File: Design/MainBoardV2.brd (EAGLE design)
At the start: 76.8 x 71.1 mm, 110 parts, among them IC1 FT230XS, T1 NDS352AP, U1 STM32F20XR, U2 MicroSDCard

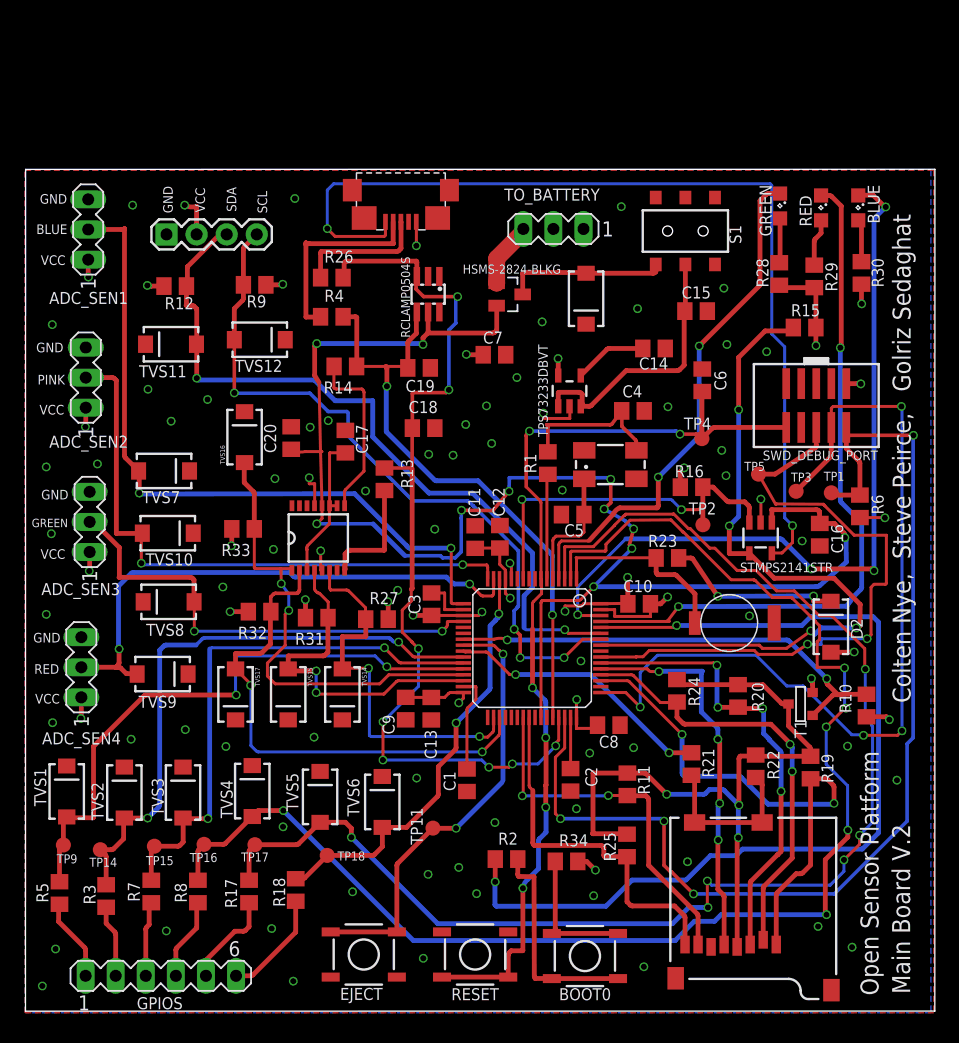
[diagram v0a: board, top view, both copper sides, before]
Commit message: Modified revision of board and schematic
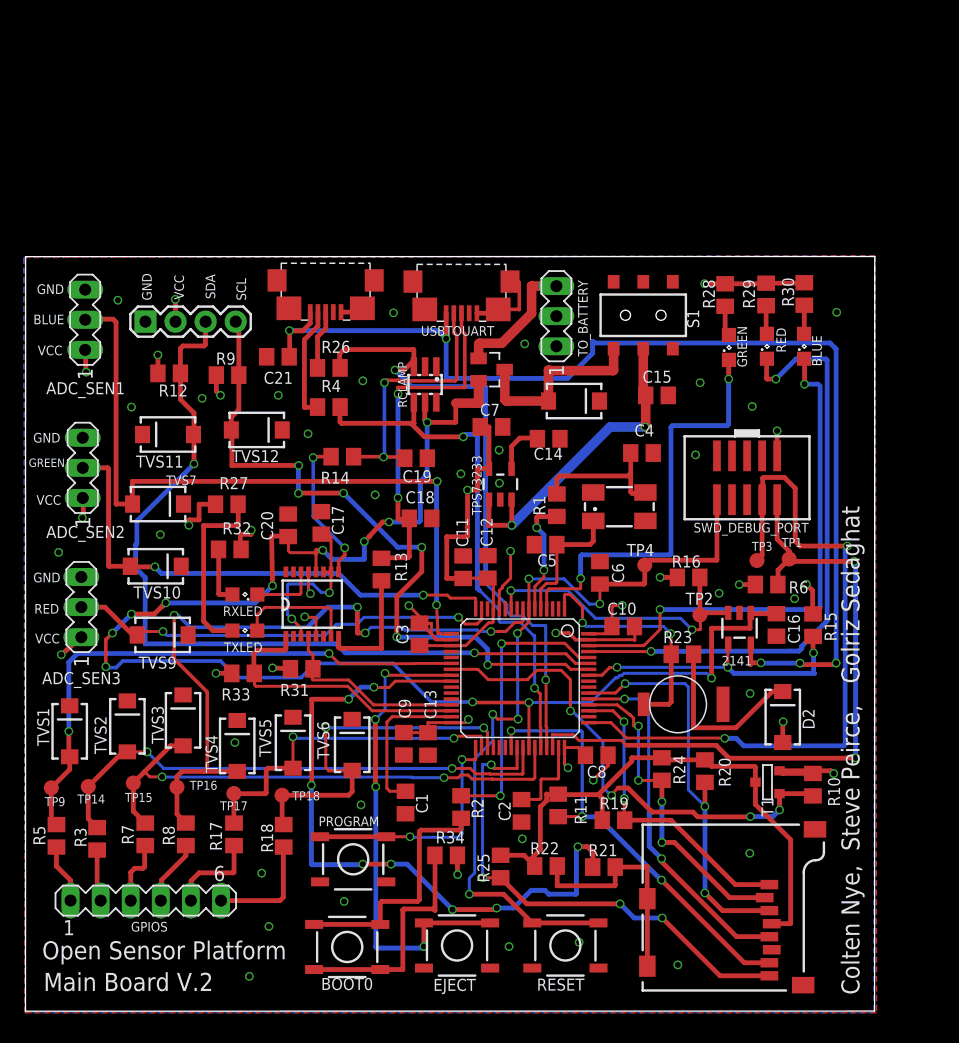
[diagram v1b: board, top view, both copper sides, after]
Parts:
- removed ADC_SEN4: (no value), con-lstb:MA03-1
- removed RCLAMP0504S: (no value), microbuilder:BREAKOUT_SOT23-6
- removed STMPS2141STR: (no value), microbuilder:SOT23-5
- removed TP11, TP5: TPB1,27, testpad:B1,27
- removed TPS73233DBVT: 3.3V, SparkFun-PowerIC:SOT23-5
- removed TVS14, TVS15, TVS16, TVS17, TVS8: TVS, SparkFun-DiscreteSemi:SMA-DIODE
- added 2141: (no value), microbuilder:SOT23-5
- added C21: 10u, rcl:C0805
- added PROGRAM: Program, SparkFun-Electromechanical:TACTILE-SWITCH-SMD
- added RCLAMP: (no value), microbuilder:BREAKOUT_SOT23-6
- added RXLED, TXLED: (no value), led:SML0805
- added TPS73233: 3.3V, SparkFun-PowerIC:SOT23-5
- added USBTOUART: USB_Shield, con-hirose:ZX62R-B-5P
- R27, R32: value 10k -> 1k
- USB_FS: value MICRO-USB-SHIELD-ZX62R-B-5P -> USB_Shield
- moved R15 25.1 mm to (66.5, 32.7), turned to 90 degrees
- moved BOOT0 20.1 mm to (27.2, 5.55), turned to 180 degrees
- moved R22 19.6 mm to (44.0, 12.4), turned to 0 degrees
- moved C6 18.4 mm to (48.5, 37.1)
- moved R19 17.2 mm to (49.7, 16.3), turned to 0 degrees
- moved R27 16.0 mm to (17.0, 42.9)
- moved U2 14.8 mm to (52.1, 1.88), turned to 270 degrees
- moved GREEN 12.7 mm to (59.4, 56.2), turned to 90 degrees
- moved RED 12.5 mm to (62.6, 56.3), turned to 90 degrees
- moved BLUE 12.5 mm to (65.7, 56.3), turned to 90 degrees
- moved R33 12.2 mm to (18.4, 28.7)
- moved C14 11.7 mm to (44.2, 48.5)
- moved TP4 11.7 mm to (52.3, 37.8)
- moved R21 11.4 mm to (48.9, 12.3), turned to 180 degrees
- moved R25 10.8 mm to (40.1, 12.3)
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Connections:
- removed net ADC1_IN0: R18.1, TP18.TP, TVS6.A, U1.14
- removed net PINK: ADC_SEN2.2, TVS10.A, U1.16
- removed net TRACESWO: SWD_DEBUG_PORT.6, TP5.TP, U1.55
- removed net USART3_CTS: IC1.6, R27.1, TVS14.A, U1.34
- removed net USART3_RTS: IC1.2, R32.1, TVS17.A, U1.35
- new net DM: C19.1, R14.1, USBTOUART.2
- new net DP: C18.1, R13.2, USBTOUART.3
- new net GPIO6: R18.1, TP18.TP, TVS6.A, U1.35
- new net N$12: R27.2, TXLED.A
- new net N$19: R32.1, RXLED.A
- new net N$22: IC1.14, RXLED.C
- new net N$23: IC1.7, TXLED.C
- new net PROGRAMMING_EN: PROGRAM.1, PROGRAM.2, U1.33
- net +3V3: now also R27.1, TPS73233.5; no longer ADC_SEN4.1, R27.2, TPS73233DBVT.5
- net DM_OUT/FS: now also RCLAMP.4; no longer C19.1, R14.1, RCLAMP0504S.4
- net DP_OUT/FS: now also RCLAMP.3; no longer C18.1, R13.2, RCLAMP0504S.3
- net GND: now also 2141.2, C21.2, PROGRAM.3, PROGRAM.4, RCLAMP.2, TPS73233.2, USBTOUART.5, USBTOUART.M1, USBTOUART.M2, USBTOUART.M3, USBTOUART.M4; no longer ADC_SEN4.3, RCLAMP0504S.2, STMPS2141STR.2, TPS73233DBVT.2, TVS14.C, TVS15.C, TVS16.C, TVS17.C, TVS8.C
- net GPIO1: now also U1.22; no longer U1.28
- net GPIO2: now also U1.41; no longer U1.26
- net GPIO3: now also U1.43; no longer U1.27
- net GPIO4: now also U1.8; no longer U1.2
- net GPIO5: now also U1.34; no longer U1.3
- net GREEN: now also ADC_SEN2.2, TVS10.A, U1.16; no longer ADC_SEN3.2, TVS8.A, U1.20
- net N$10: now also TPS73233.4; no longer TPS73233DBVT.4
- net RED: now also ADC_SEN3.2; no longer ADC_SEN4.2
- net SD_EJECT: no longer TP11.TP
- net USART3_RX: now also U1.29; no longer TVS15.A, U1.30
- net USART3_TX: now also U1.30; no longer TVS16.A, U1.29
- net USB/FS_OVERCURRENT: now also 2141.3; no longer STMPS2141STR.3
- net USB/FS_POWERSWITCHON: now also 2141.4; no longer STMPS2141STR.4
- net VBUS/FS: now also 2141.1, RCLAMP.5; no longer RCLAMP0504S.5, STMPS2141STR.1
- net VBUS/FS_IN: now also 2141.5, C21.1, USBTOUART.1; no longer STMPS2141STR.5
- net VIN: now also TPS73233.1, TPS73233.3; no longer TPS73233DBVT.1, TPS73233DBVT.3
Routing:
- net GPIO5: track 115.1 -> 29.1 mm, vias 6 -> 2
- net GPIO4: track 120.0 -> 58.5 mm, vias 6 -> 4
- net BOOT0: track 80.7 -> 24.1 mm
- net TRACESWO: track 54.2 -> 0.00 mm, vias 2 -> 0
- net PINK: track 50.7 -> 0.00 mm, vias 2 -> 0
- net USART3_RTS: track 43.1 -> 0.00 mm, vias 2 -> 0
- net ADC1_IN0: track 36.2 -> 0.00 mm, vias 2 -> 0
- net USB/FS_POWERSWITCHON: track 60.2 -> 24.7 mm, vias 4 -> 3
- net SD_DETECT: track 22.8 -> 57.9 mm, vias 2 -> 8
- net SWDIO: track 92.8 -> 57.7 mm, vias 4 -> 2
- net USART3_CTS: track 32.2 -> 0.00 mm, vias 2 -> 0
- net GPIO6: track 0.00 -> 31.3 mm, vias 0 -> 2
- net DP: track 0.00 -> 29.7 mm, vias 0 -> 2
- net DP_OUT/FS: track 78.5 -> 53.6 mm, vias 8 -> 2
- net DM: track 0.00 -> 22.6 mm, vias 0 -> 2
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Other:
- board size 76.8 x 71.1 mm -> 71.7 x 63.7 mm
- board text removed: "PINK"
